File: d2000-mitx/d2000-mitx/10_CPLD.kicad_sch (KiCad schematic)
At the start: 0 parts

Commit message: update schem + pcb layout
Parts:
- added C13, C14: 22pF, Capacitor_SMD:C_0603_1608Metric, symbol Device:C_Small
- added R10: R, symbol Device:R_Small
- added R11: NC, symbol Device:R
- added R5: 10K, Resistor_SMD:R_0402_1005Metric, symbol Device:R_Small
- added R6, R9: 1K, Resistor_SMD:R_0402_1005Metric, symbol Device:R_Small
- added R7, R8: 22R, Resistor_SMD:R_0402_1005Metric, symbol Device:R_Small
- added U13: RP2040, Package_DFN_QFN:QFN-56-1EP_7x7mm_P0.4mm_EP3.2x3.2mm, symbol MCU_RaspberryPi:RP2040
- added U4: FUSB302B01MPX, Package_DFN_QFN:WQFN-14-1EP_2.5x2.5mm_P0.5mm_EP1.45x1.45mm, symbol Interface_USB:FUSB302B01MPX
- added U8: W25Q32JVSS, Package_DFN_QFN:DFN-8-1EP_3x2mm_P0.5mm_EP1.3x1.5mm, symbol Memory_Flash:W25Q32JVSS
- added Y3: 12MHz, Crystal:Crystal_SMD_3225-4Pin_3.2x2.5mm, symbol Device:Crystal_GND24
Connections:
- new net: R5.2, R6.2, U13.56 (QSPI_SS), U8.1 (~{CS})
- new net: C13.2, U13.20 (XIN), Y3.1
- new net: U13.55 (QSPI_SD1), U8.2 (DO(IO1))
- new net: U13.54 (QSPI_SD2), U8.3 (IO2)
- new net: U13.53 (QSPI_SD0), U8.5 (DI(IO0))
- new net: U13.52 (QSPI_SCLK), U8.6 (CLK)
- new net: U13.51 (QSPI_SD3), U8.7 (IO3)
- new net: U4.12 (VCONN), U4.13 (VCONN)
- new net: R11.1, U4.2 (VBUS)
- new net: R7.1, U13.47 (USB_DP)
- new net: C14.2, R9.2, Y3.3
- new net: R9.1, U13.21 (XOUT)
- new net: R8.1, U13.46 (USB_DM)
- new net +1V0: U13.23 (DVDD), U13.45 (VREG_VOUT), U13.50 (DVDD)
- new net +3.3V: R5.1, U13.1 (IOVDD), U13.10 (IOVDD), U13.22 (IOVDD), U13.26 (RUN), U13.33 (IOVDD), U13.42 (IOVDD), U13.43 (ADC_AVDD), U13.44 (VREG_IN), U13.48 (USB_VDD), U13.49 (IOVDD), U8.8 (VCC)
- new net +3V3: R10.1, U4.3 (VDD), U4.4 (VDD)
- new net BOOT: R6.1
- new net CC1: U4.10 (CC1), U4.11 (CC1)
- new net CC2: U4.1 (CC2), U4.14 (CC2)
- new net F_INT: U13.31 (GPIO20), U4.5 (INT_N)
- new net F_SCL: U13.30 (GPIO19), U4.6 (SCL)
- new net F_SDA: U13.29 (GPIO18), U4.7 (SDA)
- new net GND: C13.1, C14.1, U13.19 (TESTEN), U13.57 (GND), U4.15 (GND), U4.8 (GND), U4.9 (GND), U8.4 (GND), Y3.2, Y3.4
- new net R_D+: R7.2
- new net R_D-: R8.2
- new net VBUS: R11.2
- new net VCONN: R10.2
- no-connect marks 0 -> 2

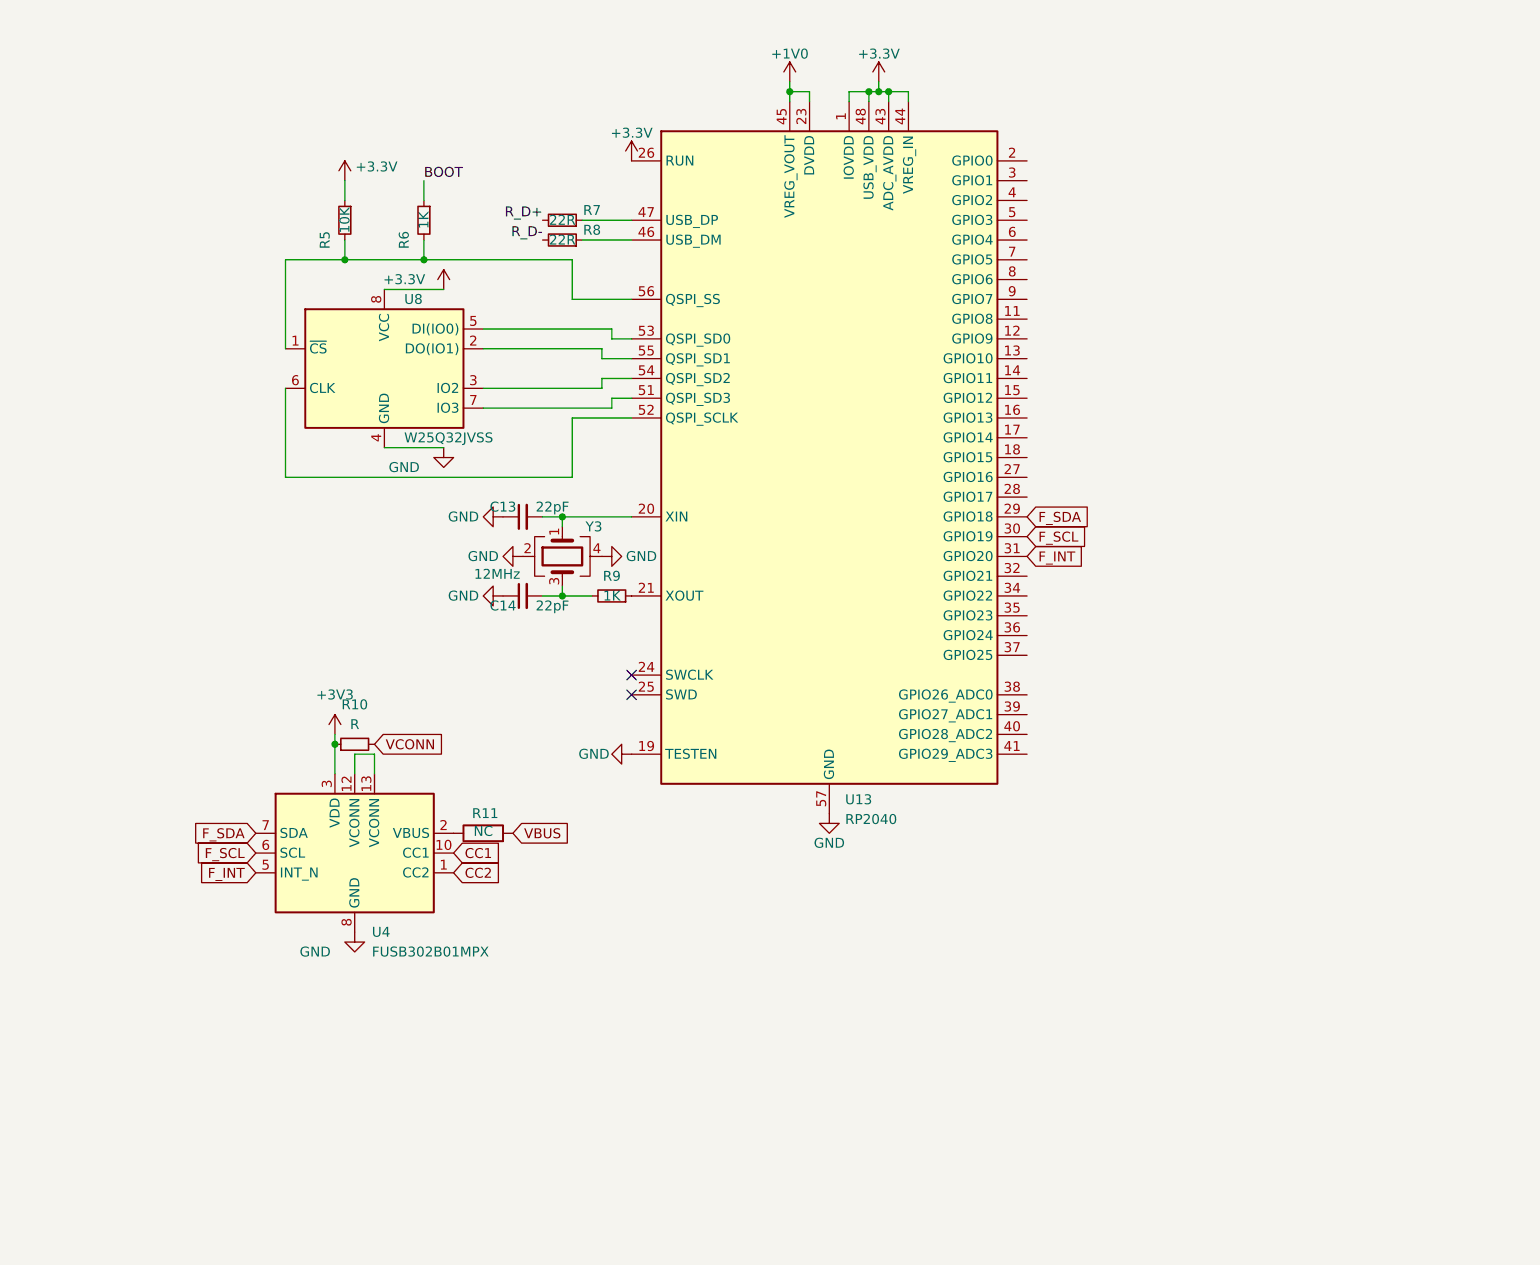
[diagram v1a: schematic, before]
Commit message: update schem + pcb layout
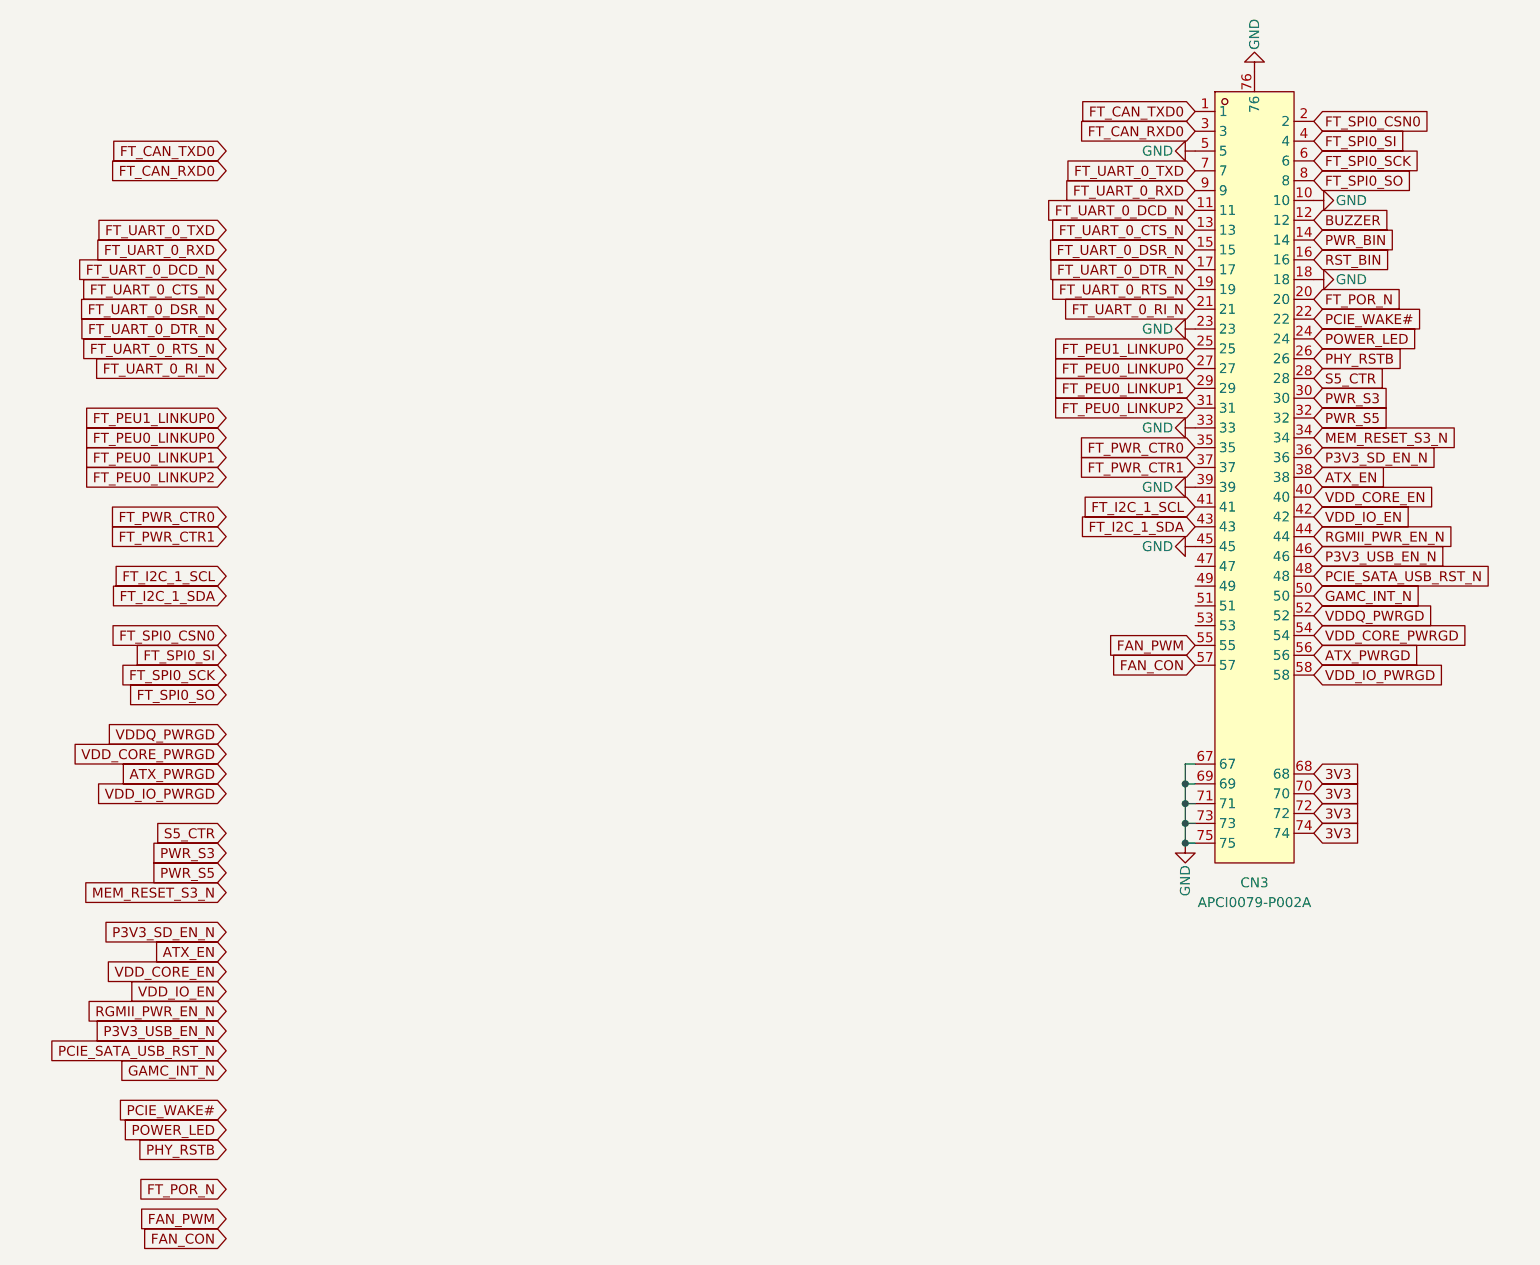
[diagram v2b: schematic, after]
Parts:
- removed C13, C14: 22pF, Capacitor_SMD:C_0603_1608Metric, symbol Device:C_Small
- removed R10: R, symbol Device:R_Small
- removed R11: NC, symbol Device:R
- removed R5: 10K, Resistor_SMD:R_0402_1005Metric, symbol Device:R_Small
- removed R6, R9: 1K, Resistor_SMD:R_0402_1005Metric, symbol Device:R_Small
- removed R7, R8: 22R, Resistor_SMD:R_0402_1005Metric, symbol Device:R_Small
- removed U13: RP2040, Package_DFN_QFN:QFN-56-1EP_7x7mm_P0.4mm_EP3.2x3.2mm, symbol MCU_RaspberryPi:RP2040
- removed U4: FUSB302B01MPX, Package_DFN_QFN:WQFN-14-1EP_2.5x2.5mm_P0.5mm_EP1.45x1.45mm, symbol Interface_USB:FUSB302B01MPX
- removed U8: W25Q32JVSS, Package_DFN_QFN:DFN-8-1EP_3x2mm_P0.5mm_EP1.3x1.5mm, symbol Memory_Flash:W25Q32JVSS
- removed Y3: 12MHz, Crystal:Crystal_SMD_3225-4Pin_3.2x2.5mm, symbol Device:Crystal_GND24
- added CN3: APCI0079-P002A, LOTES-APCI0079-P002A-M.2:PCI-SMD_APCI0079-P002A, symbol LOTES-APCI0079-P002A-M.2:APCI0079-P002A
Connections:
- net GND: now also CN3.10, CN3.18, CN3.23, CN3.33, CN3.39, CN3.45, CN3.5, CN3.67, CN3.69, CN3.71, CN3.73, CN3.75, CN3.76
- new net 3V3: CN3.68, CN3.70, CN3.72, CN3.74
- new net ATX_EN: CN3.38
- new net ATX_PWRGD: CN3.56
- new net BUZZER: CN3.12
- new net FAN_CON: CN3.57
- new net FAN_PWM: CN3.55
- new net FT_CAN_RXD0: CN3.3
- new net FT_CAN_TXD0: CN3.1
- new net FT_I2C_1_SCL: CN3.41
- new net FT_I2C_1_SDA: CN3.43
- new net FT_PEU0_LINKUP0: CN3.27
- new net FT_PEU0_LINKUP1: CN3.29
- new net FT_PEU0_LINKUP2: CN3.31
- new net FT_PEU1_LINKUP0: CN3.25
- new net FT_POR_N: CN3.20
- new net FT_PWR_CTR0: CN3.35
- new net FT_PWR_CTR1: CN3.37
- new net FT_SPI0_CSN0: CN3.2
- new net FT_SPI0_SCK: CN3.6
- new net FT_SPI0_SI: CN3.4
- new net FT_SPI0_SO: CN3.8
- new net FT_UART_0_CTS_N: CN3.13
- new net FT_UART_0_DCD_N: CN3.11
- new net FT_UART_0_DSR_N: CN3.15
- new net FT_UART_0_DTR_N: CN3.17
- new net FT_UART_0_RI_N: CN3.21
- new net FT_UART_0_RTS_N: CN3.19
- new net FT_UART_0_RXD: CN3.9
- new net FT_UART_0_TXD: CN3.7
- new net GAMC_INT_N: CN3.50
- new net MEM_RESET_S3_N: CN3.34
- new net P3V3_SD_EN_N: CN3.36
- new net P3V3_USB_EN_N: CN3.46
- new net PCIE_SATA_USB_RST_N: CN3.48
- new net PCIE_WAKE#: CN3.22
- new net PHY_RSTB: CN3.26
- new net POWER_LED: CN3.24
- new net PWR_BIN: CN3.14
- new net PWR_S3: CN3.30
- new net PWR_S5: CN3.32
- new net RGMII_PWR_EN_N: CN3.44
- new net RST_BIN: CN3.16
- new net S5_CTR: CN3.28
- new net VDDQ_PWRGD: CN3.52
- new net VDD_CORE_EN: CN3.40
- new net VDD_CORE_PWRGD: CN3.54
- new net VDD_IO_EN: CN3.42
- new net VDD_IO_PWRGD: CN3.58
- no-connect marks 2 -> 0
